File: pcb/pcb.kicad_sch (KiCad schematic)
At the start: 20 parts, among them U1 STM32F103C8T6

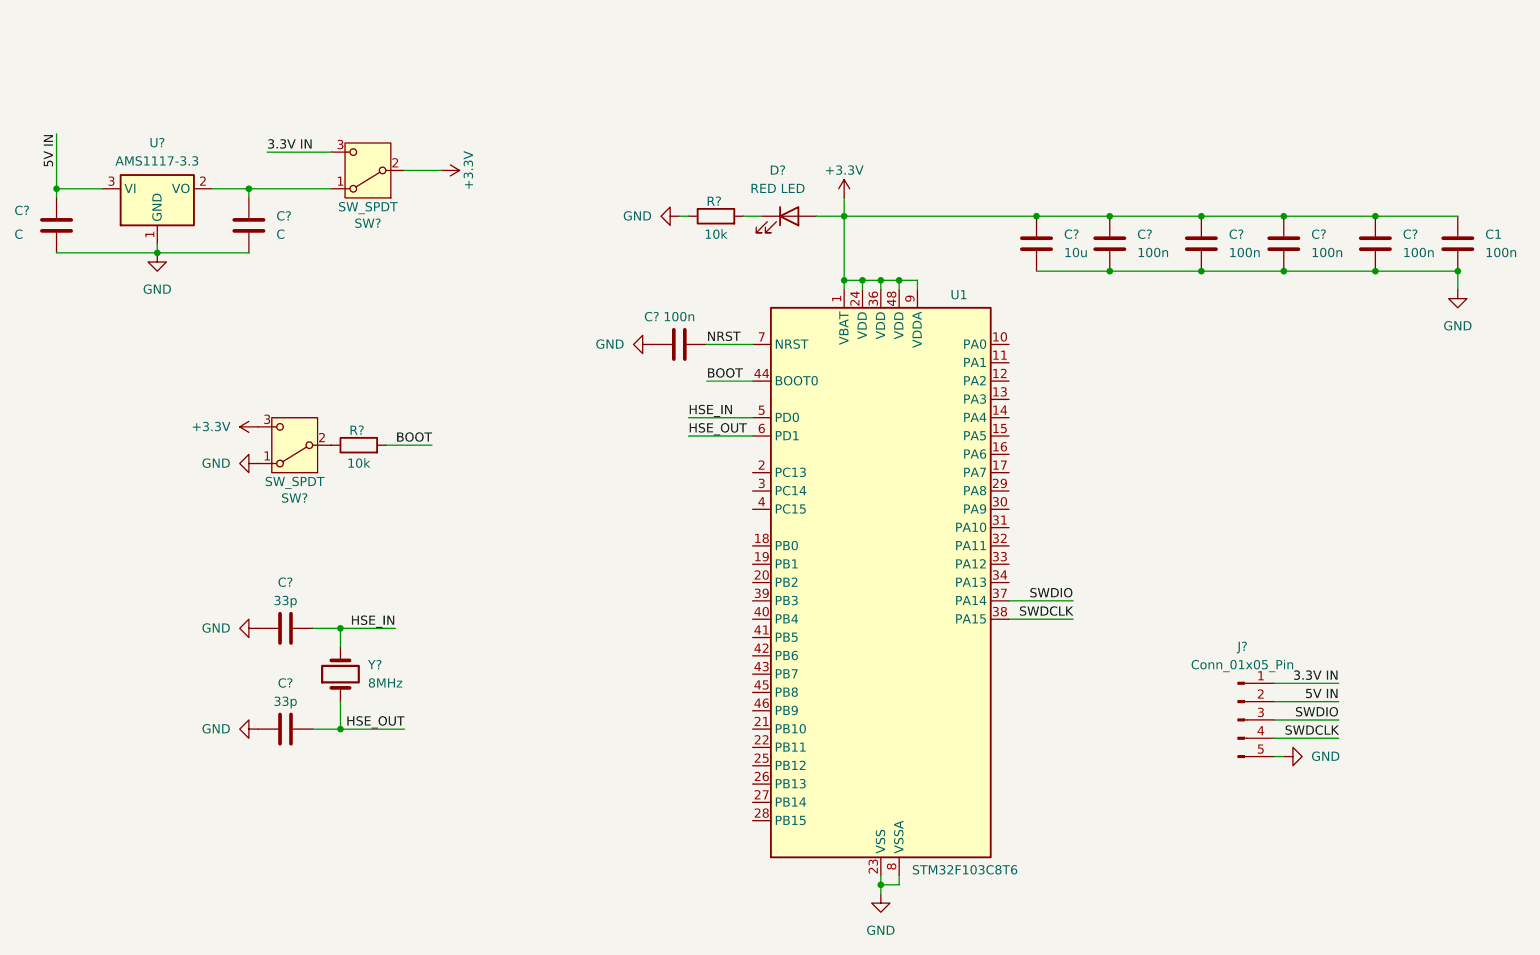
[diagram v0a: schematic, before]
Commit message: Change kicad version to 9.0.7
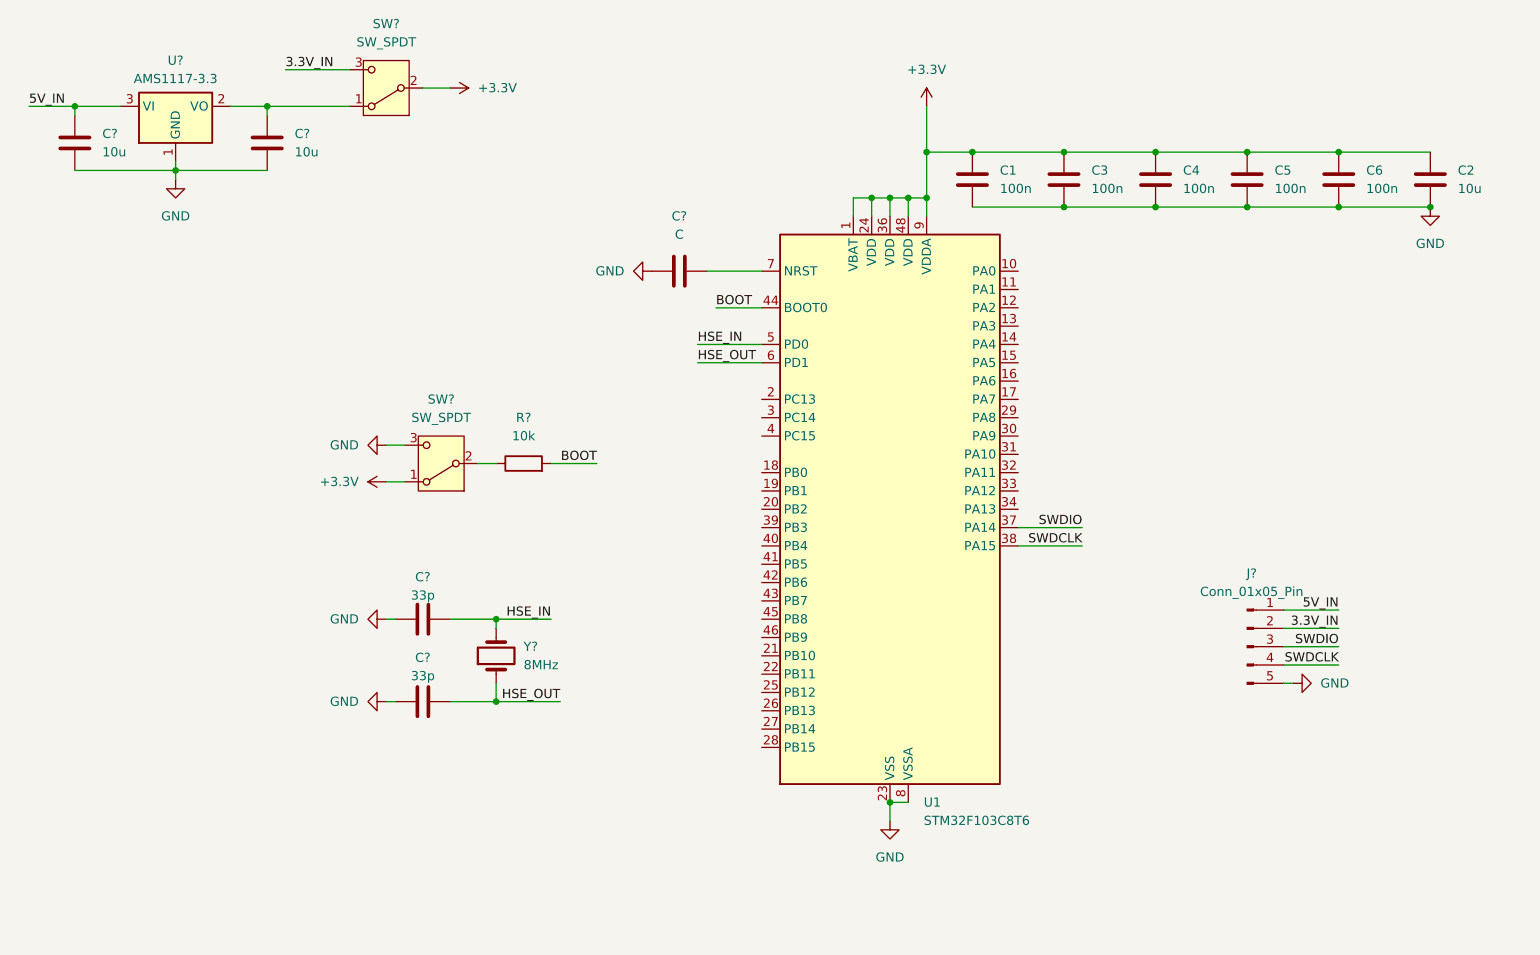
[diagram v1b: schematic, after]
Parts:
- removed C? (x2): C, symbol Device:C
- removed C? (x5): 100n, symbol Device:C
- removed C? (x2): 33p, symbol Device:C
- removed C?: 10u, symbol Device:C
- removed D?: RED LED, symbol Device:LED
- removed J?: Conn_01x05_Pin, symbol Connector:Conn_01x05_Pin
- removed R? (x2): 10k, symbol Device:R
- removed SW? (x2): SW_SPDT, symbol Switch:SW_SPDT
- removed U?: AMS1117-3.3, Package_TO_SOT_SMD:SOT-223-3_TabPin2, symbol Regulator_Linear:AMS1117-3.3
- removed Y?: 8MHz, symbol Device:Crystal
- added C2, C? (x2): 10u, symbol Device:C
- added C3, C4, C5, C6: 100n, symbol Device:C
- added C? (x2): 33p, symbol Device:C
- added C?: C, symbol Device:C
- added J?: Conn_01x05_Pin, symbol Connector:Conn_01x05_Pin
- added R?: 10k, symbol Device:R
- added SW? (x2): SW_SPDT, symbol Switch:SW_SPDT
- added U?: AMS1117-3.3, Package_TO_SOT_SMD:SOT-223-3_TabPin2, symbol Regulator_Linear:AMS1117-3.3
- added Y?: 8MHz, symbol Device:Crystal
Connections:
- net +3.3V: now also C2.1, C3.1, C4.1, C5.1, C6.1, SW?.1 (A), SW?.2 (B)
- net BOOT: now also R?.2
- net GND: now also C2.2, C3.2, C4.2, C5.2, C6.2, C?.1, C?.1, C?.1, C?.2, C?.2, J?.5 (Pin_5), SW?.3 (C), U?.1 (GND)
- net HSE_IN: now also C?.2, Y?.2
- net HSE_OUT: now also C?.2, Y?.1
- net SWDCLK: now also J?.4 (Pin_4)
- net SWDIO: now also J?.3 (Pin_3)
- net NRST: no longer names the net of U1.7 (NRST)
- net NRST: now also C?.2
- new net: C?.1, SW?.1 (A), U?.2 (VO)
- new net: R?.1, SW?.2 (B)
- new net 3.3V_IN: J?.2 (Pin_2), SW?.3 (C)
- new net 5V_IN: C?.1, J?.1 (Pin_1), U?.3 (VI)
